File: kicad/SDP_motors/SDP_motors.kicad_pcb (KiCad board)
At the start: 4 copper layers, 98 x 98 mm, 76 parts, among them J1 Conn_01x04, J10 MOTOR, J2 Conn_01x04, J3 Conn_01x04, J4 Conn_01x04, J5 Conn_01x04, J6 Conn_01x04, J7 Conn_01x02, J8 Conn_01x02, J9 Conn_01x02, Q1 IRLZ44N, Q2 IRLZ44N, Q3 IRLZ44N

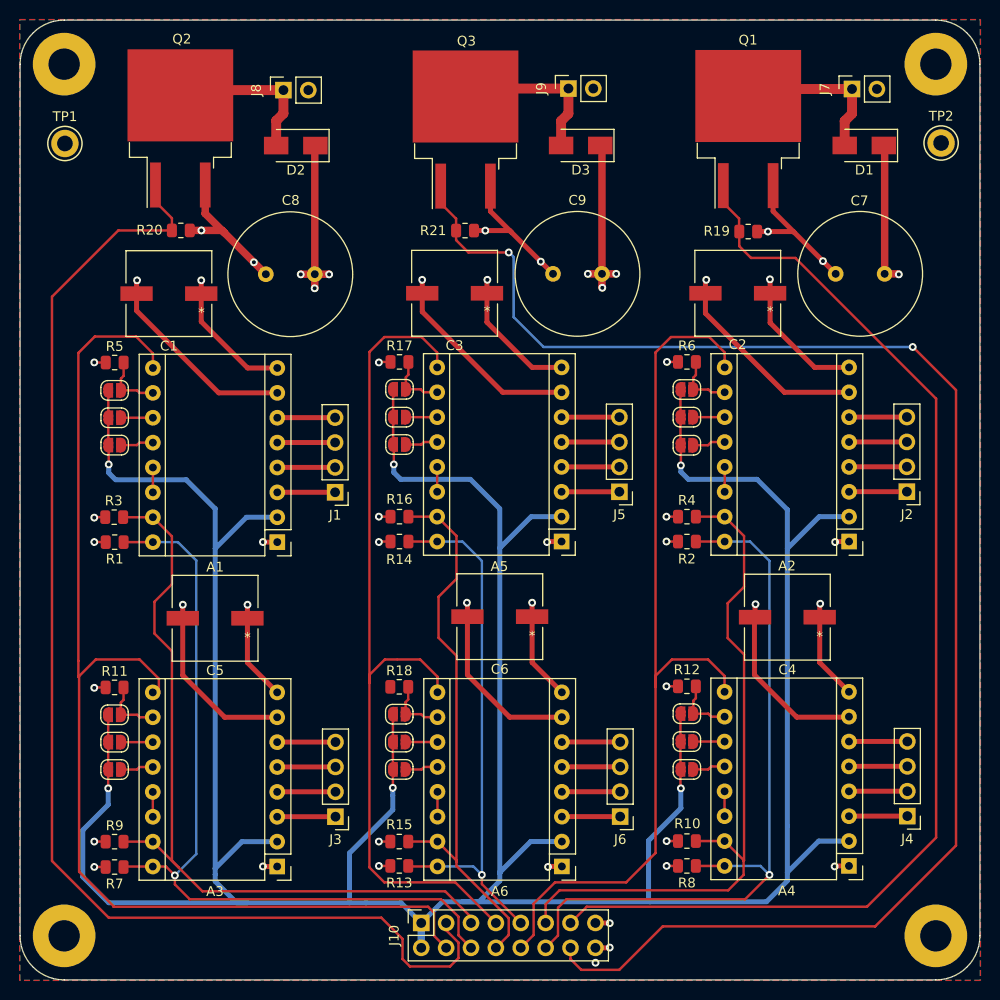
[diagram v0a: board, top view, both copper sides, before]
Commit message: Final PCB layout changes
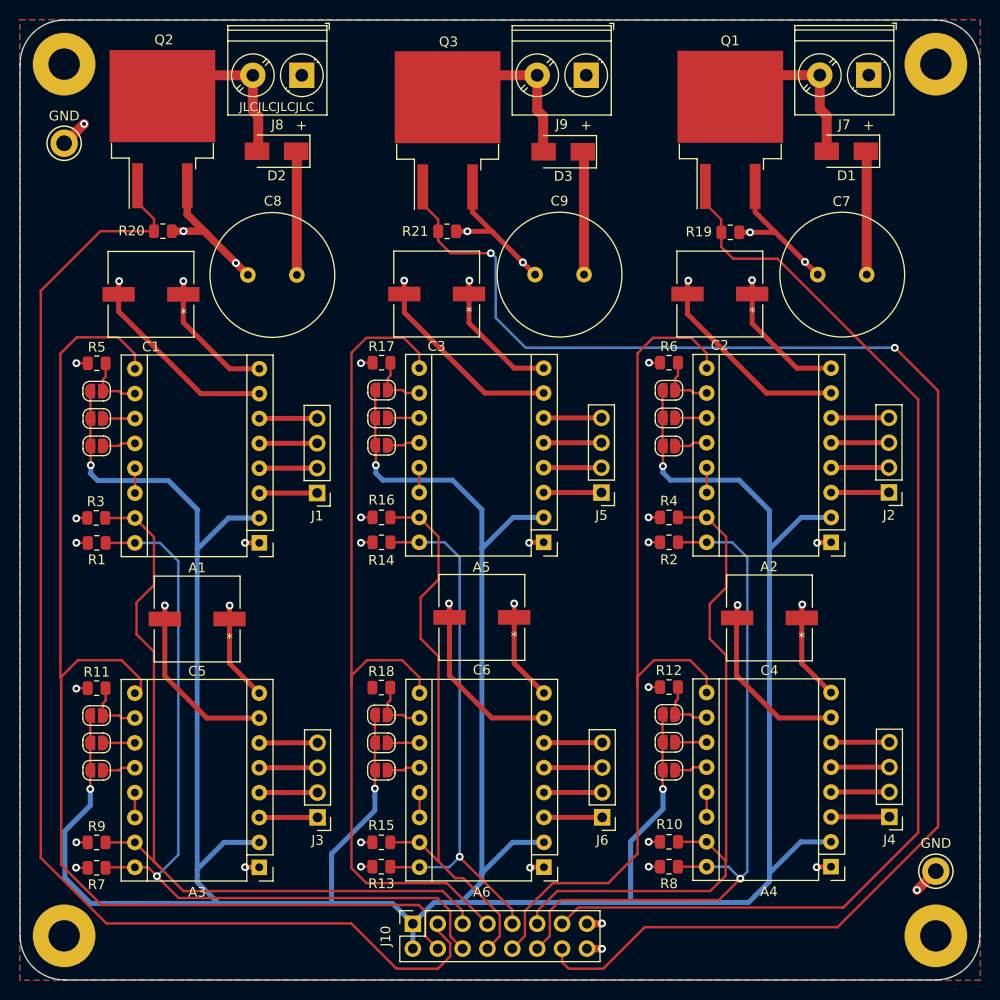
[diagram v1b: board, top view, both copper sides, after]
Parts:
- J7, J8, J9: footprint Connector_PinSocket_2.54mm:PinSocket_1x02_P2.54mm_Vertical -> TerminalBlock_Phoenix:TerminalBlock_Phoenix_PT-1,5-2-5.0-H_1x02_P5.00mm_Horizontal
- moved TP2 74.3 mm to (179.4, 133.7)
- moved J8 2.41 mm to (114.7, 52.4), turned to 180 degrees
- moved J9 2.26 mm to (143.7, 52.4), turned to 180 degrees
- moved J7 2.22 mm to (172.6, 52.4), turned to 180 degrees
- moved D2 2.04 mm to (112.1, 60.2)
- moved D1 1.92 mm to (170.3, 60.2)
- moved D3 1.89 mm to (141.4, 60.2)
- moved A6 1.83 mm to (139.4, 133.3)
- moved R10 1.83 mm to (152.2, 130.7)
- moved R7 1.83 mm to (93.7, 133.4)
- moved R9 1.83 mm to (93.7, 130.8)
- moved C2 1.83 mm to (157.4, 74.8)
- moved C3 1.83 mm to (128.5, 74.8)
- moved C7 1.83 mm to (172.4, 72.8)
- moved C9 1.83 mm to (143.5, 72.8)
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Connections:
- J7 pad 1: Net-(D1-Pad2) -> +12V
- J7 pad 2: +12V -> Net-(D1-Pad2)
- J8 pad 1: Net-(D2-Pad2) -> +12V
- J8 pad 2: +12V -> Net-(D2-Pad2)
- J9 pad 1: Net-(D3-Pad2) -> +12V
- J9 pad 2: +12V -> Net-(D3-Pad2)
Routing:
- net +12V: track 124.2 -> 113.8 mm, vias 14 -> 7
- net GND: track 196.6 -> 202.0 mm, vias 37 -> 38
- net P84_DIR: track 75.9 -> 72.9 mm
- net P88_MTR2: track 159.9 -> 157.7 mm
- net Net-(D2-Pad2): track 16.7 -> 15.1 mm
- net P72_FAN: track 129.6 -> 128.2 mm
- net P77_STEP: track 80.6 -> 82.0 mm
- net P83_STEP: track 70.9 -> 69.5 mm
- net P82_EN: track 91.8 -> 90.5 mm
- net P87_MTR1: track 119.2 -> 117.8 mm
- net Net-(D3-Pad2): track 17.0 -> 18.2 mm
- net Net-(D1-Pad2): track 17.0 -> 18.1 mm
- net P80_STEP: track 57.9 -> 58.9 mm
- net P79_EN: track 88.3 -> 89.3 mm
- net P78_DIR: track 81.8 -> 82.7 mm
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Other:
- board text added: "+"
- board text added: "GND"
- board text added: "JLCJLCJLCJLC"
